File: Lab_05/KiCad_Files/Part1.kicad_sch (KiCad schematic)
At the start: 9 parts, among them Q10 NPN

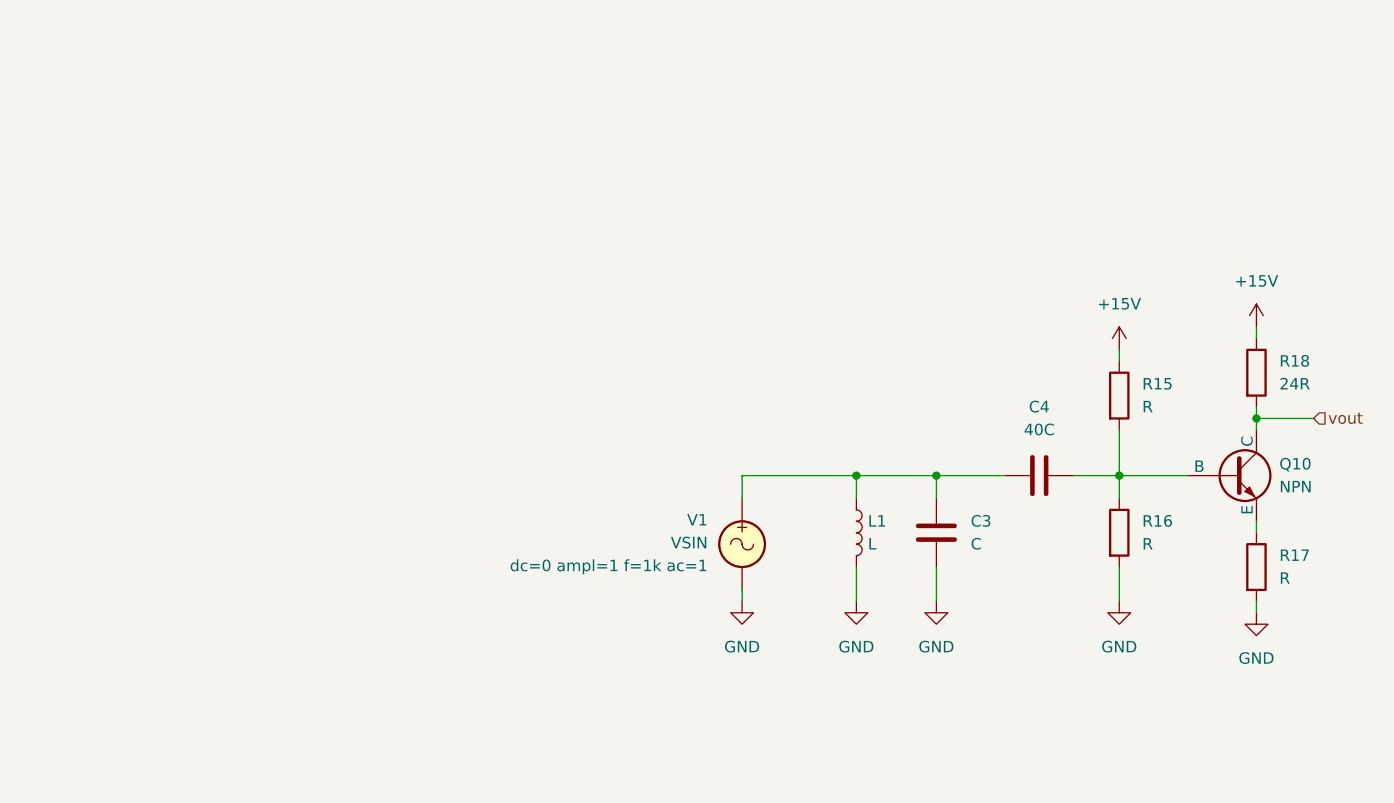
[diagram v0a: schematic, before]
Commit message: Continue Lab 5
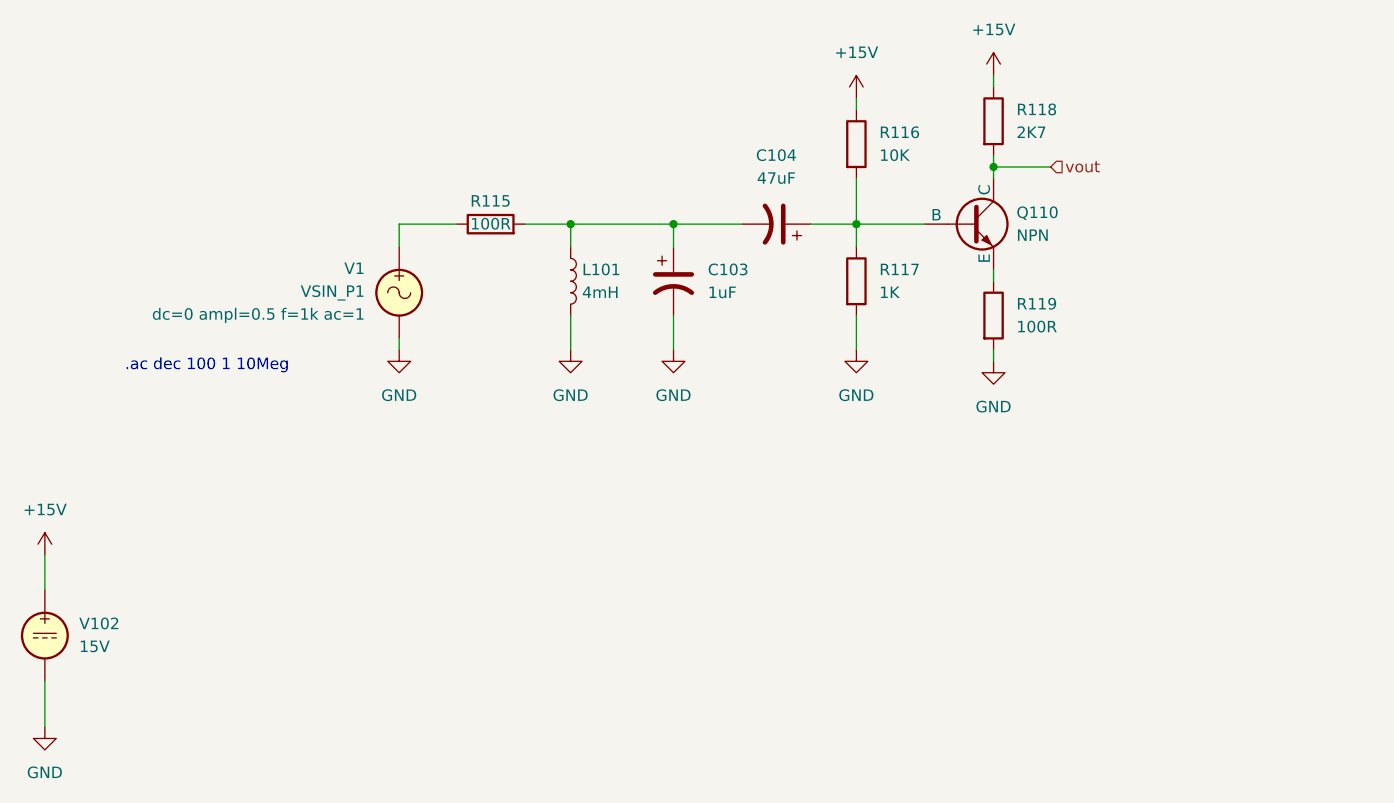
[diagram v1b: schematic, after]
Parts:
- added R115: 100R, symbol Device:R
- added V102: 15V, symbol Simulation_SPICE:VDC
- C103: renamed from C3; value C -> 1uF; symbol Device:C -> Device:C_Polarized_US
- C104: renamed from C4; value 40C -> 47uF; symbol Device:C -> Device:C_Polarized_US
- L101: renamed from L1; value L -> 4mH
- R116: renamed from R15; value R -> 10K
- R117: renamed from R16; value R -> 1K
- R118: renamed from R18; value 24R -> 2K7
- R119: renamed from R17; value R -> 100R
- V1: value VSIN -> VSIN_P1
- renumbered Q10 to Q110
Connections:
- net +15V: now also V102.1
- net GND: now also V102.2
- net at Q110.2 (B), R116.2, R117.1: now also C104.1; no longer C104.2
- net at C103.1, L101.1: now also C104.2, R115.2; no longer C104.1, V1.1
- new net: R115.1, V1.1
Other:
- note added: ".ac dec 100 1 10Meg"
- company: (none) -> Jim Horwitz & Mark Vaughn, Jork Incorporated
- title: (none) -> Single-Transistor Bandpass Amplifier
- moved on the sheet: L101, Q110, R116, R117, R118, R119
